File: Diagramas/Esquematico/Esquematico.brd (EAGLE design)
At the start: 70 x 80.1 mm, 48 parts, among them IC3 DS3231N_DIP, IC4 3071_SMD, J1 Modulo Pir, J2 RASPBERRYPI-40-PIN-GPIO_SMT, K1 SRD-05VDC-SL-C, K2 SRD-05VDC-SL-C, K3 SRD-05VDC-SL-C, K4 SRD-05VDC-SL-C, U1 RFM69HW-868S2

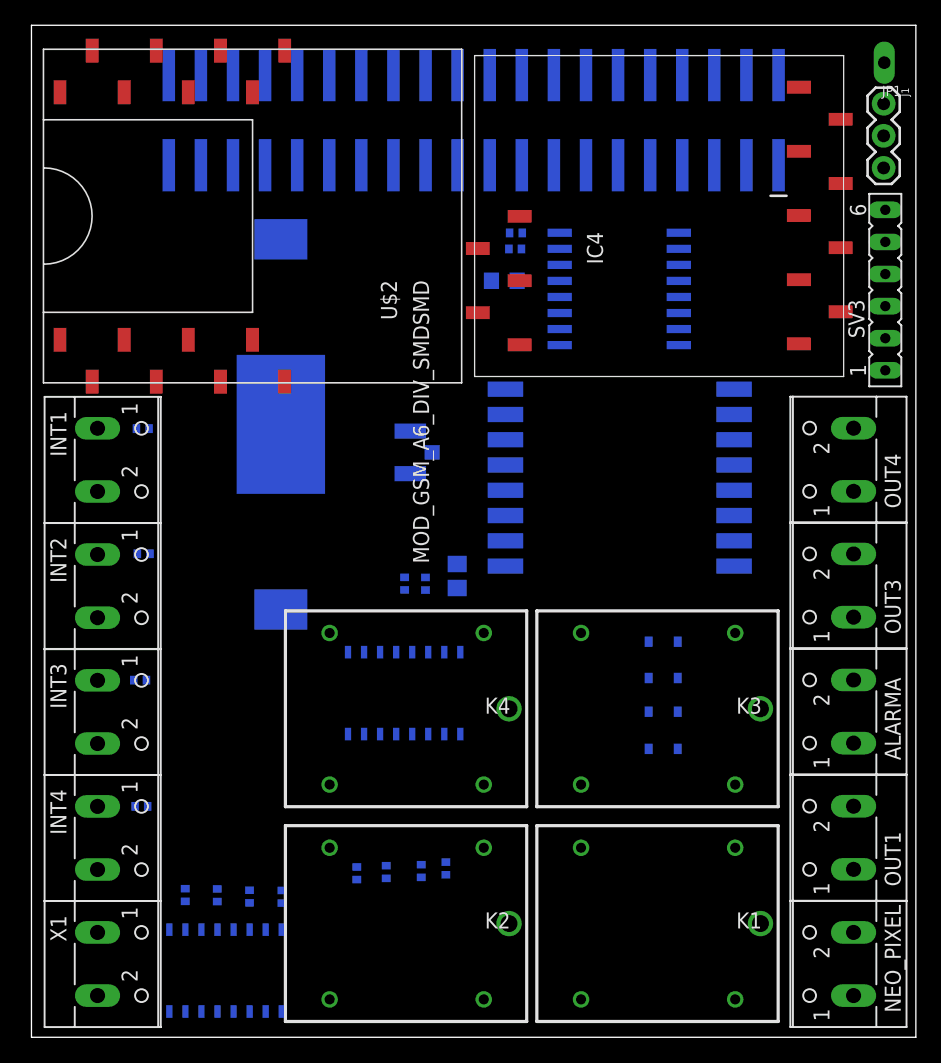
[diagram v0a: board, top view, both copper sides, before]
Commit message: Ruteado de los componentes
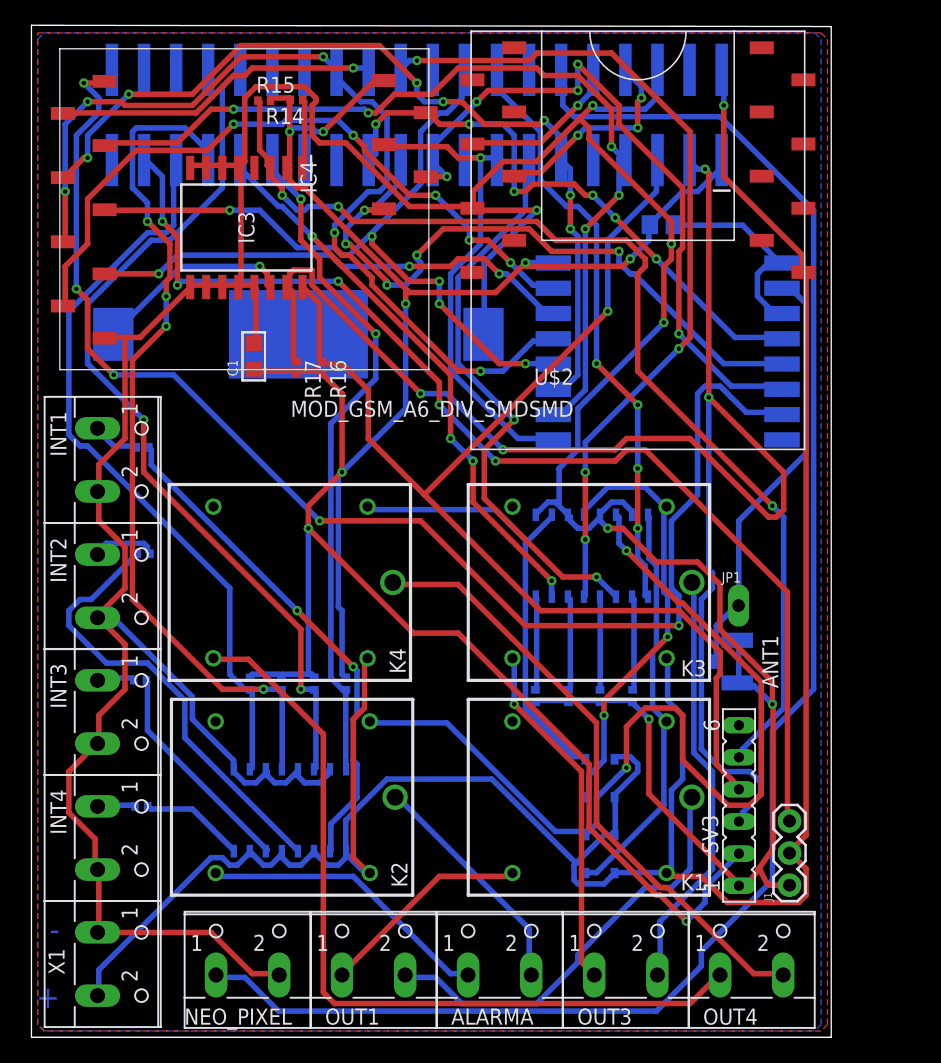
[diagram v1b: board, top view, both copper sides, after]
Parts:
- moved J1 62.3 mm to (60.0, 12.0), turned to 90 degrees
- moved NEO_PIXEL 46.7 mm to (17.1, 6.20), turned to 0 degrees
- moved JP1 44.5 mm to (56.0, 34.2), turned to 0 degrees
- moved SV3 42.4 mm to (56.0, 18.4)
- moved R15 40.3 mm to (18.4, 74.1), flipped to the top, turned to 0 degrees
- moved OUT4 40.1 mm to (57.0, 6.20), turned to 0 degrees
- moved R14 39.2 mm to (21.0, 74.2), flipped to the top, turned to 180 degrees
- moved OUT1 38.0 mm to (27.1, 6.20), turned to 0 degrees
- moved OUT3 34.0 mm to (47.0, 6.20), turned to 0 degrees
- moved ALARMA 33.1 mm to (37.1, 6.20), turned to 0 degrees
- moved IC4 32.8 mm to (16.9, 65.5), turned to 270 degrees
- moved C3 32.2 mm to (49.9, 64.3), turned to 180 degrees
- moved ANT1 30.7 mm to (55.9, 29.7), turned to 90 degrees
- moved U$2 30.6 mm to (48.0, 63.1), turned to 90 degrees
- moved IC3 29.9 mm to (17.0, 64.1), flipped to the top, turned to 270 degrees
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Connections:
- net 5V: now also J1.2; no longer J1.3
- net INT5: now also J1.3; no longer J1.2
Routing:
- net GND: track 0.00 -> 340.5 mm, vias 0 -> 7
- net 5V: track 0.00 -> 196.3 mm, vias 0 -> 1
- net 3.3V: track 0.00 -> 186.8 mm, vias 0 -> 8
- net G18: track 0.00 -> 130.7 mm
- net SDA: track 0.00 -> 125.6 mm, vias 0 -> 4
- net CS: track 0.00 -> 107.5 mm, vias 0 -> 5
- net SCL: track 0.00 -> 95.7 mm, vias 0 -> 1
- net INT5: track 0.00 -> 89.7 mm, vias 0 -> 5
- net SQW: track 0.00 -> 85.4 mm, vias 0 -> 3
- net G3: track 0.00 -> 75.0 mm, vias 0 -> 5
- net N$34: track 0.00 -> 74.8 mm, vias 0 -> 2
- net G0: track 0.00 -> 71.8 mm, vias 0 -> 5
- net G1: track 0.00 -> 70.4 mm, vias 0 -> 7
- net INT2: track 0.00 -> 69.4 mm, vias 0 -> 2
- net INT3: track 0.00 -> 68.1 mm, vias 0 -> 4
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- added copper zone on layer 16, net GND
- added copper zone on layer 1, net GNG
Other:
- board size 70 x 80.1 mm -> 63.3 x 80.1 mm
- board text added: "+"
- board text added: "-"
